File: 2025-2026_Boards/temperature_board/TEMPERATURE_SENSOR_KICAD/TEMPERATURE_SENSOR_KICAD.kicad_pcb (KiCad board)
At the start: 2 copper layers, 72 parts, among them J1 LCD Connector Pinout, J10 Conn_01x02_Pin, J11 Conn_01x02_Pin, J12 Conn_01x02_Pin, J13 Conn_01x02_Pin, J14 Conn_01x02_Pin, J15 Conn_01x02_Pin, J16 Conn_01x02_Pin, J17 Conn_01x02_Pin, J18 Conn_01x02_Pin, J19 Conn_01x02_Pin, J2 Conn_01x02_Pin, J20 Conn_01x02_Pin, J21 Conn_01x02_Pin, J24 Conn_01x03_Socket, J25 Conn_01x03_Socket, J3 Conn_01x02_Pin, J4 Conn_01x02_Pin, J5 Conn_01x02_Pin, J6 Conn_01x02_Pin, J7 Conn_01x02_Pin, J8 Conn_01x02_Pin, J9 Conn_01x02_Pin, U1 STM32G431CBT6, U2 TMP235A4DBZR, U3 AMS1117-3.3, U4 TCAN1057AEV-Q1, U5 TPS62932DRLR, U6 TPS62932DRLR, U8 AMS1117

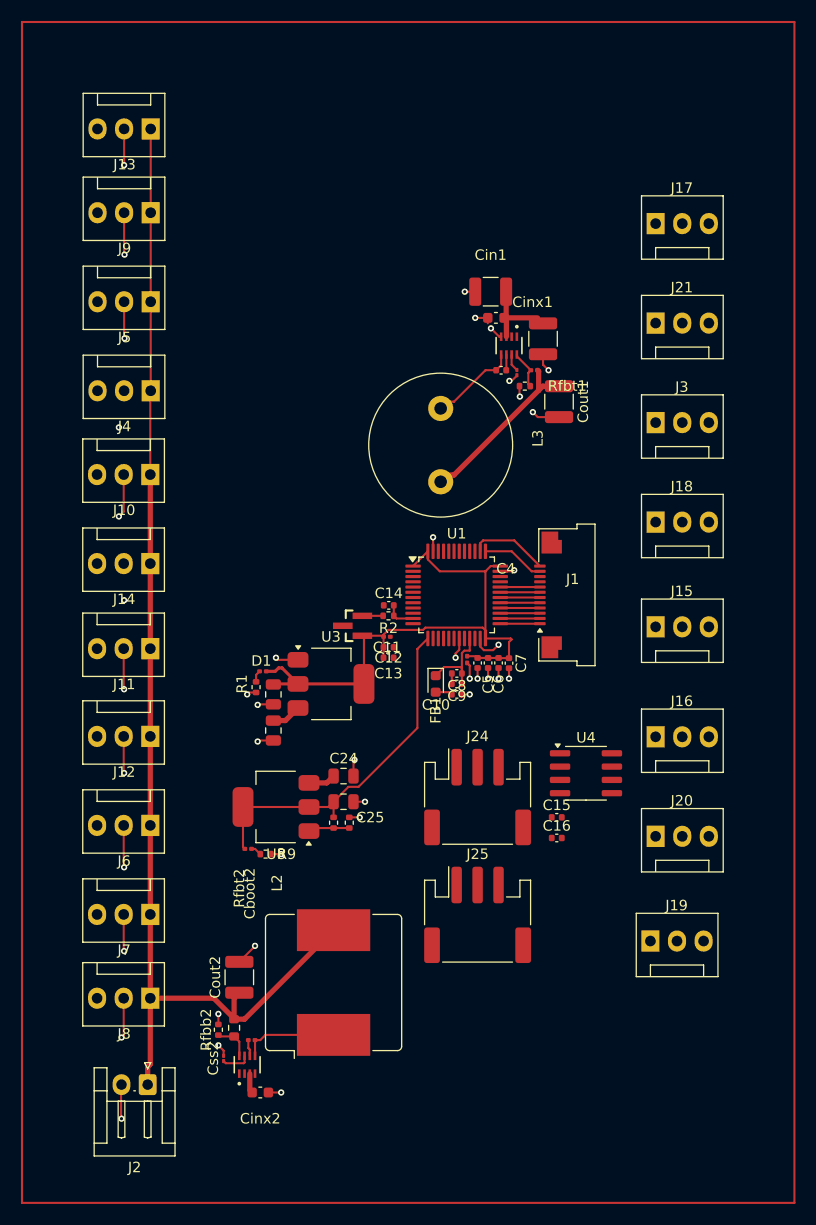
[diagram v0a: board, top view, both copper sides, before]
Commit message: finishing the board. debuggign,ectc
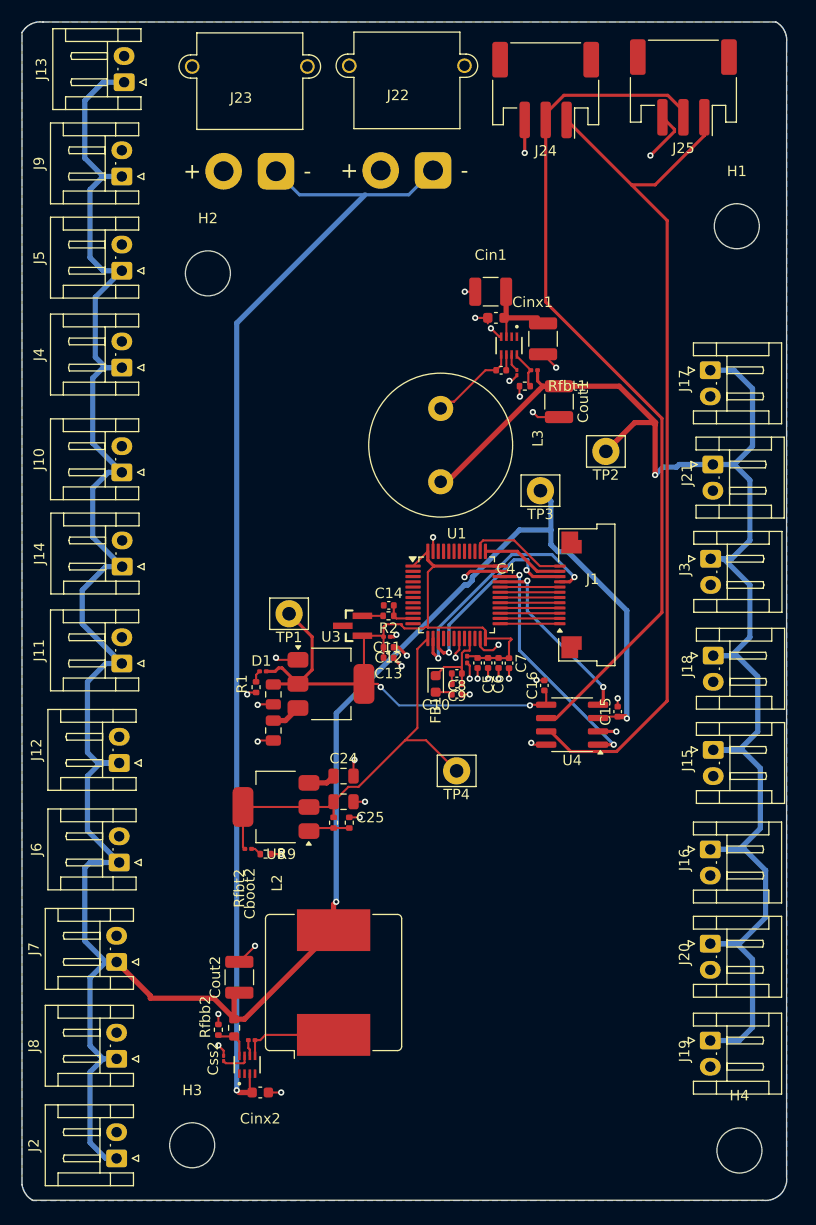
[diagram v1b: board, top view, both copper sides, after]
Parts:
- added H1: MountingHole, MountingHole:MountingHole_4.3mm_M4, F.Cu at (139.5, 88.8)
- added H2: MountingHole, MountingHole:MountingHole_4.3mm_M4, F.Cu at (89.0, 93.2)
- added H3: MountingHole, MountingHole:MountingHole_4.3mm_M4, F.Cu at (87.5, 176.5)
- added H4: MountingHole, MountingHole:MountingHole_4.3mm_M4, F.Cu at (139.8, 177.0)
- added J22: Conn_01x02_Pin, Connector_AMASS:AMASS_XT30PW-M_1x02_P2.50mm_Horizontal, F.Cu at (110.5, 83.4)
- added J23: Conn_01x02_Pin, Connector_AMASS:AMASS_XT30PW-M_1x02_P2.50mm_Horizontal, F.Cu at (95.5, 83.5)
- added TP1: TestPoint, Connector_Pin:Pin_D1.3mm_L10.0mm_W3.5mm_Flat, F.Cu at (96.8, 125.8)
- added TP2: TestPoint, Connector_Pin:Pin_D1.3mm_L10.0mm_W3.5mm_Flat, F.Cu at (127.0, 110.2)
- added TP3: TestPoint, Connector_Pin:Pin_D1.3mm_L10.0mm_W3.5mm_Flat, F.Cu at (120.8, 114.0)
- added TP4: TestPoint, Connector_Pin:Pin_D1.3mm_L10.0mm_W3.5mm_Flat, F.Cu at (112.8, 140.8)
- J10, J11, J12, J13, J14, J15, J16, J17, J18, J19, J20, J21, J3, J4, J5, J6, J7, J8, J9: footprint Connector:FanPinHeader_1x03_P2.54mm_Vertical -> Connector_JST:JST_EH_S2B-EH_1x02_P2.50mm_Horizontal
- moved J25 81.4 mm to (134.4, 75.5), turned to 180 degrees
- moved J24 67.8 mm to (121.2, 75.8), turned to 180 degrees
- moved J17 14.9 mm to (137.0, 102.5), turned to -90 degrees
- moved C16 14.6 mm to (121.1, 132.6), turned to 90 degrees
- moved J21 14.6 mm to (137.2, 111.5), turned to -90 degrees
- moved J3 14.0 mm to (137.0, 120.5), turned to -90 degrees
- moved J18 13.9 mm to (137.2, 129.8), turned to -90 degrees
- moved J15 13.0 mm to (137.2, 138.8), turned to -90 degrees
- moved J16 11.9 mm to (137.0, 148.2), turned to -90 degrees
- moved C15 11.7 mm to (128.1, 135.1), turned to 90 degrees
- moved J20 11.5 mm to (137.0, 157.2), turned to -90 degrees
- moved J19 11.1 mm to (137.0, 166.5), turned to -90 degrees
- moved J2 7.64 mm to (80.3, 177.8), turned to 90 degrees
- moved J8 6.62 mm to (80.3, 168.2), turned to 90 degrees
- moved J7 5.56 mm to (80.3, 159.0), turned to 90 degrees
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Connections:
- C16 pad 1: 3.3 -> +3.3V
- U4 pad 5: 3.3 -> +3.3V
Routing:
- net 12V: track 17.0 -> 150.0 mm, vias 0 -> 1
- net 5V: track 122.2 -> 254.2 mm, vias 0 -> 2
- net 28V: track 10.3 -> 119.3 mm, vias 0 -> 1
- net CAN+: track 0.00 -> 84.4 mm
- net CAN-: track 0.00 -> 82.6 mm
- net +3.3V: track 57.6 -> 85.7 mm, vias 0 -> 2
- net Net-(J1-Pin_9): track 0.00 -> 23.4 mm, vias 0 -> 2
- net FDCAN_TX: track 0.00 -> 23.3 mm, vias 0 -> 2
- net Net-(J1-Pin_10): track 0.00 -> 19.4 mm, vias 0 -> 2
- net GND: track 78.6 -> 59.6 mm, vias 41 -> 38
- net FDCAN_RX: track 0.00 -> 17.7 mm, vias 0 -> 2
- net +2.2V: track 34.3 -> 40.4 mm
- net Net-(J1-Pin_8): track 3.79 -> 5.69 mm
- net Net-(J1-Pin_7): track 3.79 -> 5.69 mm
- net Net-(J1-Pin_6): track 3.79 -> 5.69 mm
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- added copper zone on B.Cu, net GND
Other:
- board outline added: 73 x 112.5 mm
